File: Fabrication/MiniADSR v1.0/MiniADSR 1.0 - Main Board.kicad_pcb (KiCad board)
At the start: 2 copper layers, 105 x 128.5 mm, 50 parts, among them J1 INPUT, J2 OUTPUT, J3 JST_BUS, J4 ControlBoard_Pins, J5 IDC_BUS, J6 MainBoard_Pins, Q1 BC547, Q2 BC547, Q3 BC547, U1 LM555, U2 TL072

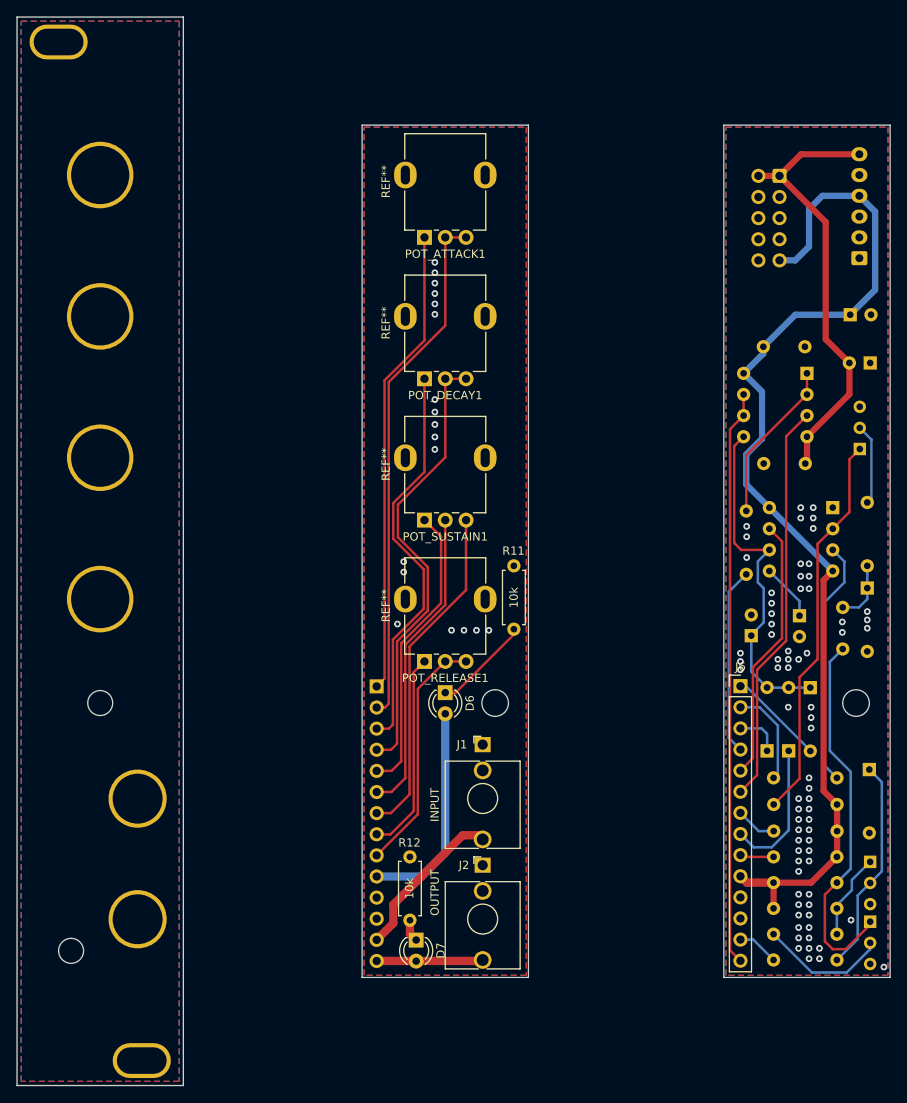
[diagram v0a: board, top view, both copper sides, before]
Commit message: Added fabrication files
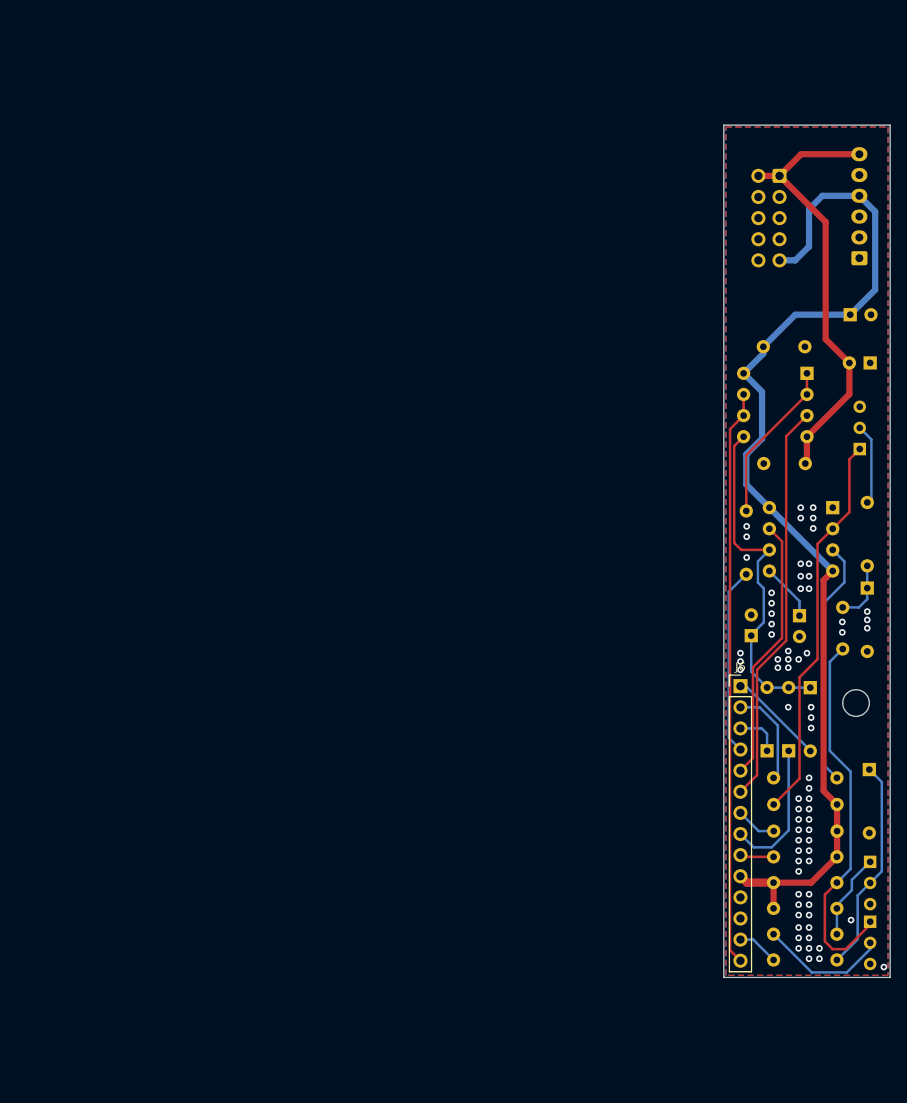
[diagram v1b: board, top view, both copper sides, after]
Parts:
- removed D6: PWR_LED, LED_THT:LED_D3.0mm
- removed D7: OUTPUT_LED, LED_THT:LED_D3.0mm
- removed J1: INPUT, benjiaomodular:AudioJack_3.5mm
- removed J2: OUTPUT, benjiaomodular:AudioJack_3.5mm
- removed J4: ControlBoard_Pins, Connector_PinSocket_2.54mm:PinSocket_1x14_P2.54mm_Vertical
- removed POT_ATTACK1, POT_DECAY1, POT_RELEASE1, POT_SUSTAIN1: 1M, benjiaomodular:Potentiometer_RV09
- removed R11, R12: 10k, Resistor_THT:R_Axial_DIN0207_L6.3mm_D2.5mm_P7.62mm_Horizontal
- removed the REF** at (64.5, 127.5)
- removed the REF** at (107.5, 122.5)
- removed the REF** at (57.5, 117.5)
- removed the REF** at (57.5, 100.5)
- removed the REF** at (57.5, 83.5)
- removed the REF** at (57.5, 66.5)
- removed the REF** at (50.0, 40.0)
- removed the REF** at (64.5, 142.0)
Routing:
- net A4: track 63.0 -> 0.00 mm
- net A3: track 56.4 -> 0.00 mm
- net A6: track 54.5 -> 0.00 mm
- net A5: track 48.3 -> 0.00 mm
- net A9: track 40.7 -> 0.00 mm
- net A8: track 37.2 -> 0.00 mm
- net A7: track 35.2 -> 0.00 mm
- net A11: track 29.2 -> 0.00 mm
- net A_VCC: track 26.1 -> 0.00 mm
- net A10: track 24.2 -> 0.00 mm
- net A1: track 19.3 -> 0.00 mm
- net A2: track 12.8 -> 0.00 mm
- net Net-(D6-Pad1): track 11.8 -> 0.00 mm
- net Net-(D7-Pad1): track 2.69 -> 0.00 mm
- net GND1: vias 18 -> 0
- removed copper zone on B.Cu, net (none)
- removed copper zone on F.Cu, net (none)
- removed copper zone on B.Cu, net GND1
- removed copper zone on F.Cu, net GND1
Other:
- board size 105 x 128.5 mm -> 20 x 102.5 mm
- board text removed: "@benjiaomodular"
- board text removed: "A"
- board text removed: "D"
- board text removed: "IN"
- board text removed: "MiniADSR"
- board text removed: "OUT"
- board text removed: "R"
- board text removed: "S"
